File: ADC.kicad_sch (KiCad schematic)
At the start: 16 parts, among them J3 ANALOG VOLTAGE INPUTS, J8 CURRENT INPUTS, J9 DIFFERENTIAL INPUTS, U12 REF3333, U13 ADS1261

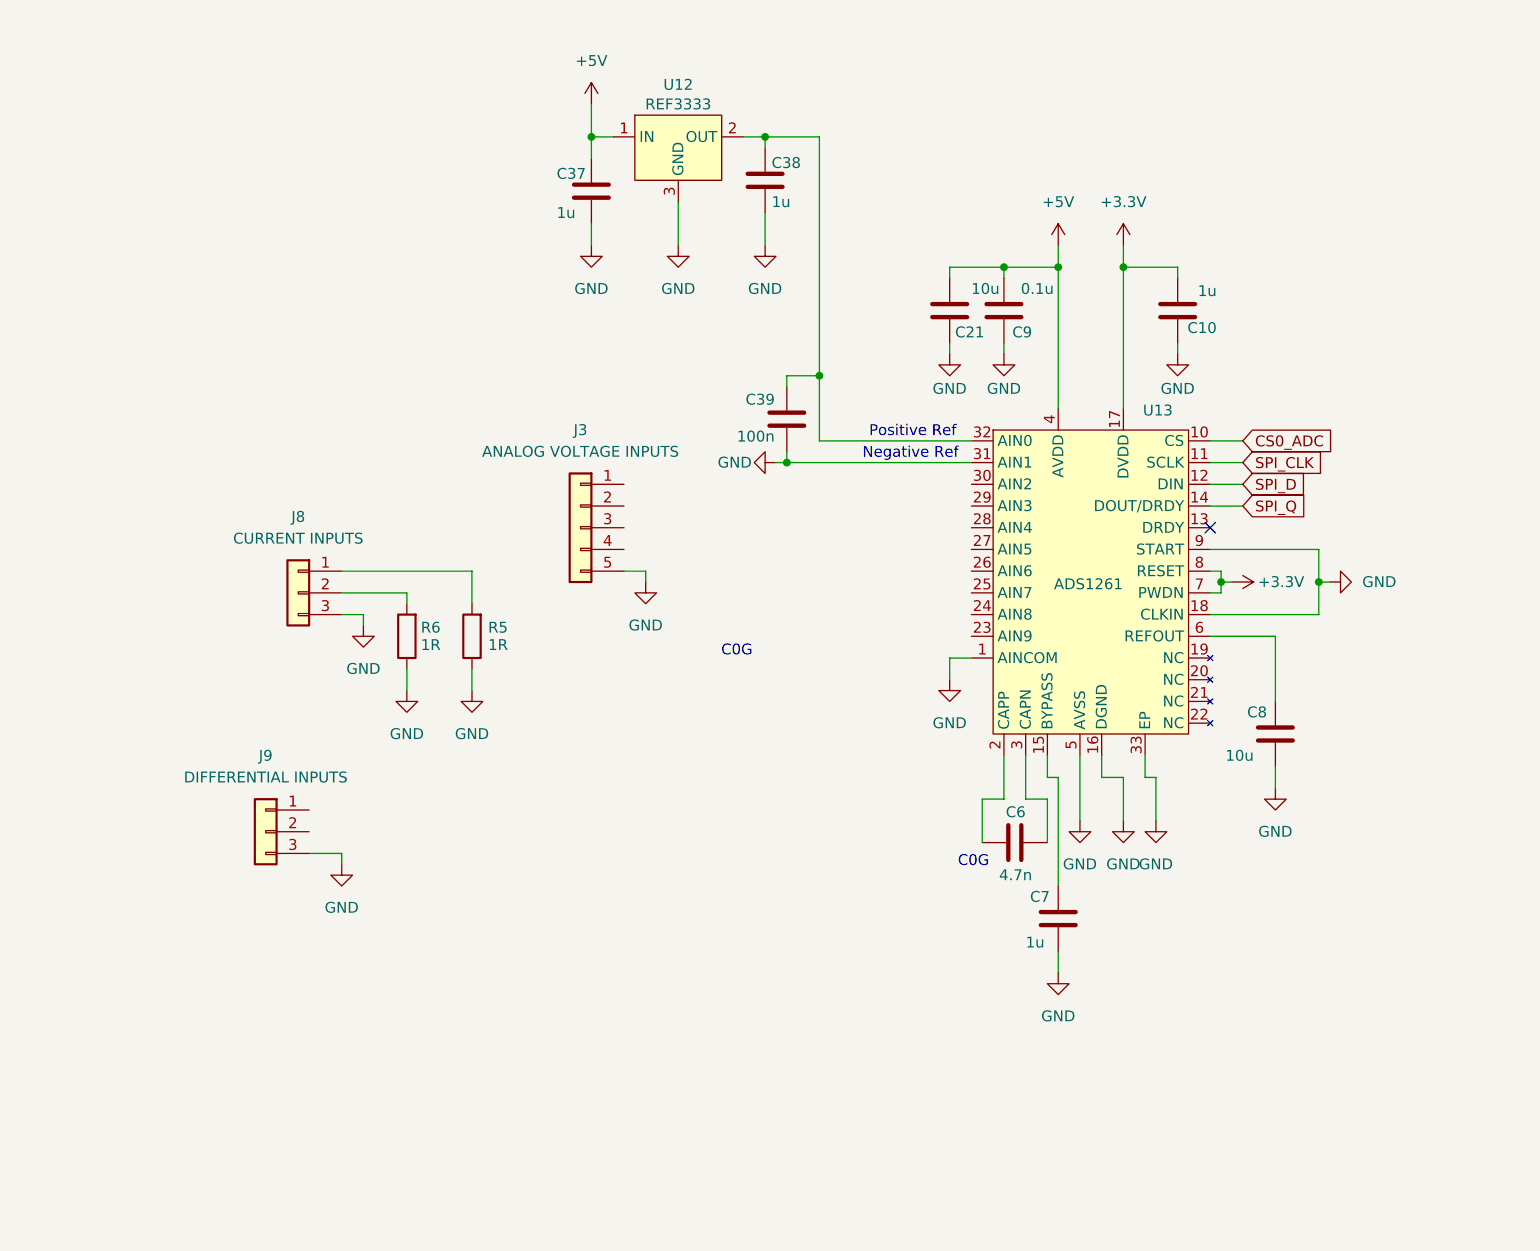
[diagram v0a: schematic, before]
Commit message: 9/18/2026 schematic work
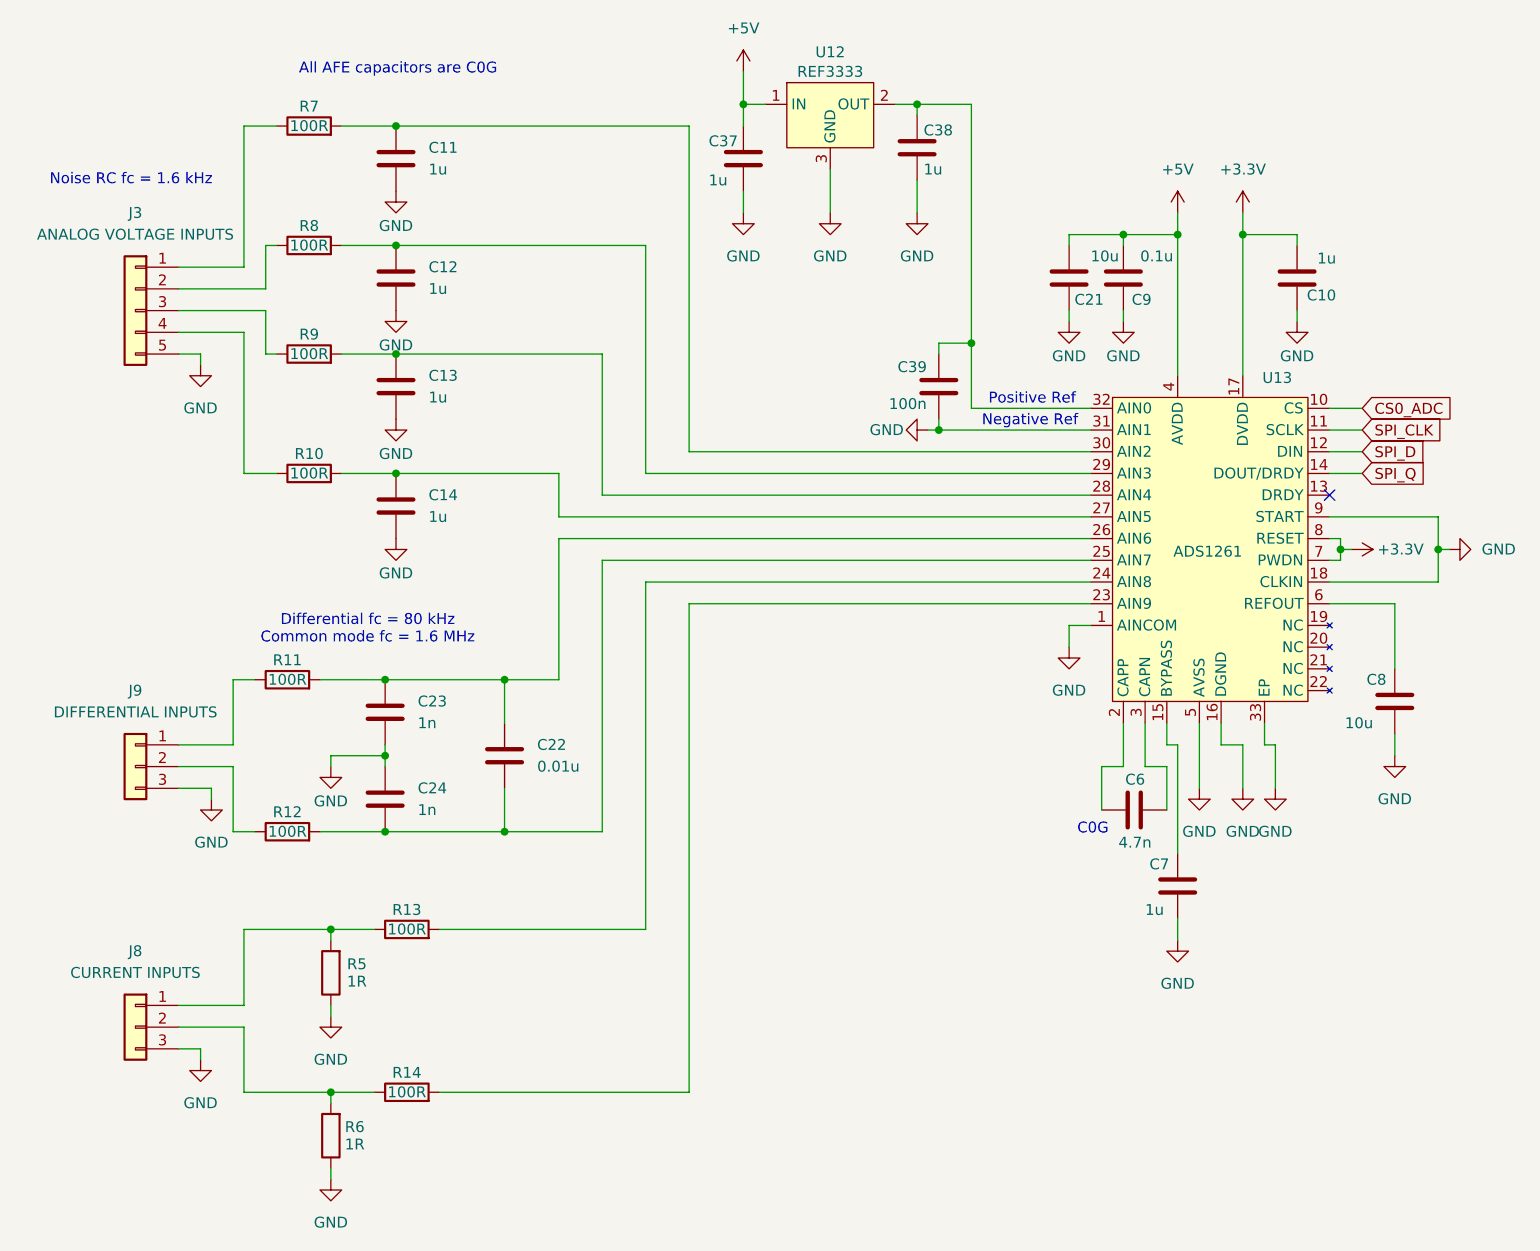
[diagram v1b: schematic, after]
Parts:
- added C11, C12, C13, C14: 1u, symbol Device:C
- added C22: 0.01u, symbol Device:C
- added C23, C24: 1n, symbol Device:C
- added R10, R11, R12, R13, R14, R7, R8, R9: 100R, symbol Device:R
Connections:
- net GND: now also C11.2, C12.2, C13.2, C14.2, C23.2, C24.1
- net at J8.2 (Pin_2), R6.2: now also R14.1
- net at J8.1 (Pin_1), R5.2: now also R13.1
- net at J9.1 (Pin_1): now also R11.1
- net at J9.2 (Pin_2): now also R12.1
- net at J3.1 (Pin_1): now also R7.1
- net at J3.2 (Pin_2): now also R8.1
- net at J3.3 (Pin_3): now also R9.1
- net at J3.4 (Pin_4): now also R10.1
- net at U13.23 (AIN9): now also R14.2
- net at U13.24 (AIN8): now also R13.2
- net at U13.25 (AIN7): now also C22.2, C24.2, R12.2
- net at U13.26 (AIN6): now also C22.1, C23.1, R11.2
- net at U13.27 (AIN5): now also C14.1, R10.2
- net at U13.28 (AIN4): now also C13.1, R9.2
- net at U13.29 (AIN3): now also C12.1, R8.2
- net at U13.30 (AIN2): now also C11.1, R7.2
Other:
- note added: "All AFE capacitors are C0G"
- note added: "Differential fc = 80 kHz Common mode fc = 1.6 MHz"
- note added: "Noise RC fc = 1.6 kHz"
- moved on the sheet: C10, C21, C37, C38, C39, C6, C7, C8, C9, J3, J8, J9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
